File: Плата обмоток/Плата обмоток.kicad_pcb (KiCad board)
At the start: 2 copper layers, 58 x 58 mm, 20 parts, among them J1 4900, J10 4900, J11 4900, J12 4900, J13 4900, J14 A1, J15 A2, J16 B1, J17 B2, J18 C1, J19 C2, J2 4900, J3 4900, J4 Conn_01x02, J5 Conn_02x02_Odd_Even, J6 Conn_01x02, J7 Conn_01x02, J8 4900, J9 4900

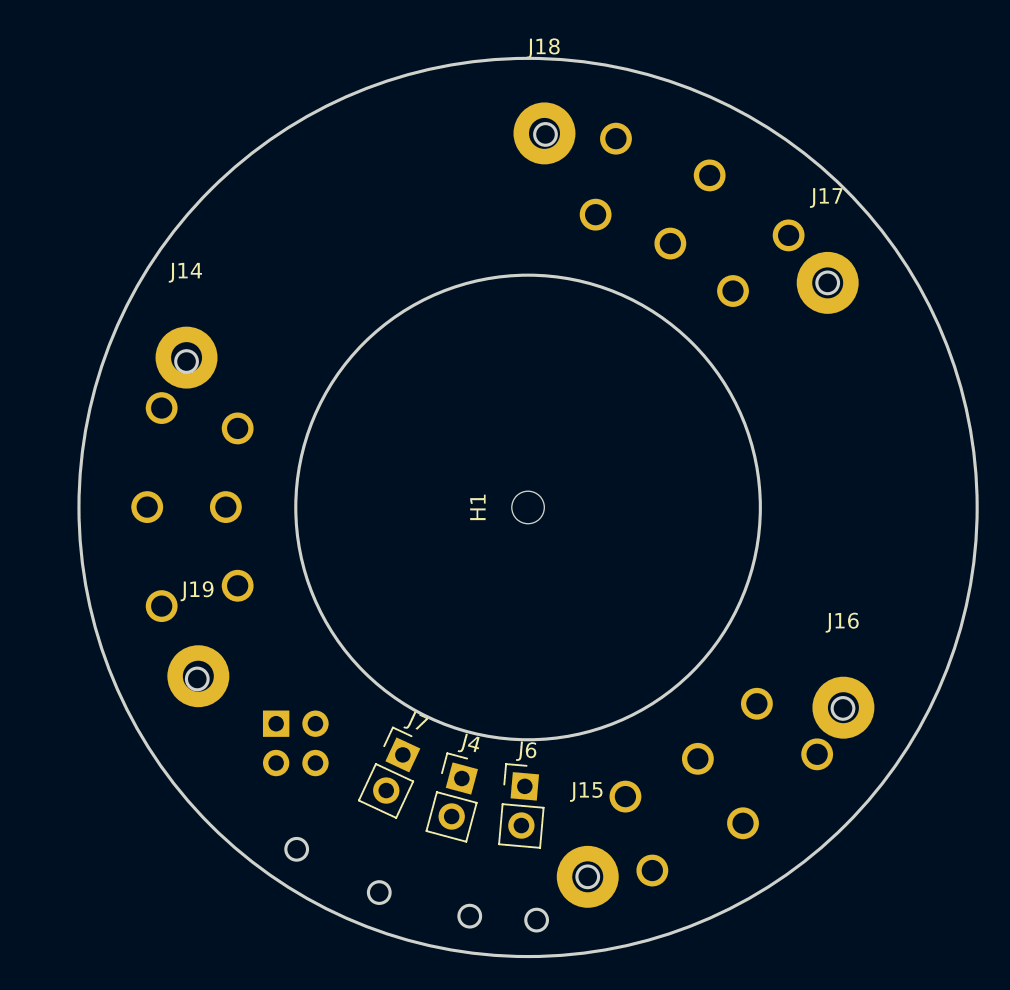
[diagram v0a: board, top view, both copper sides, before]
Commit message: Финальная доработка
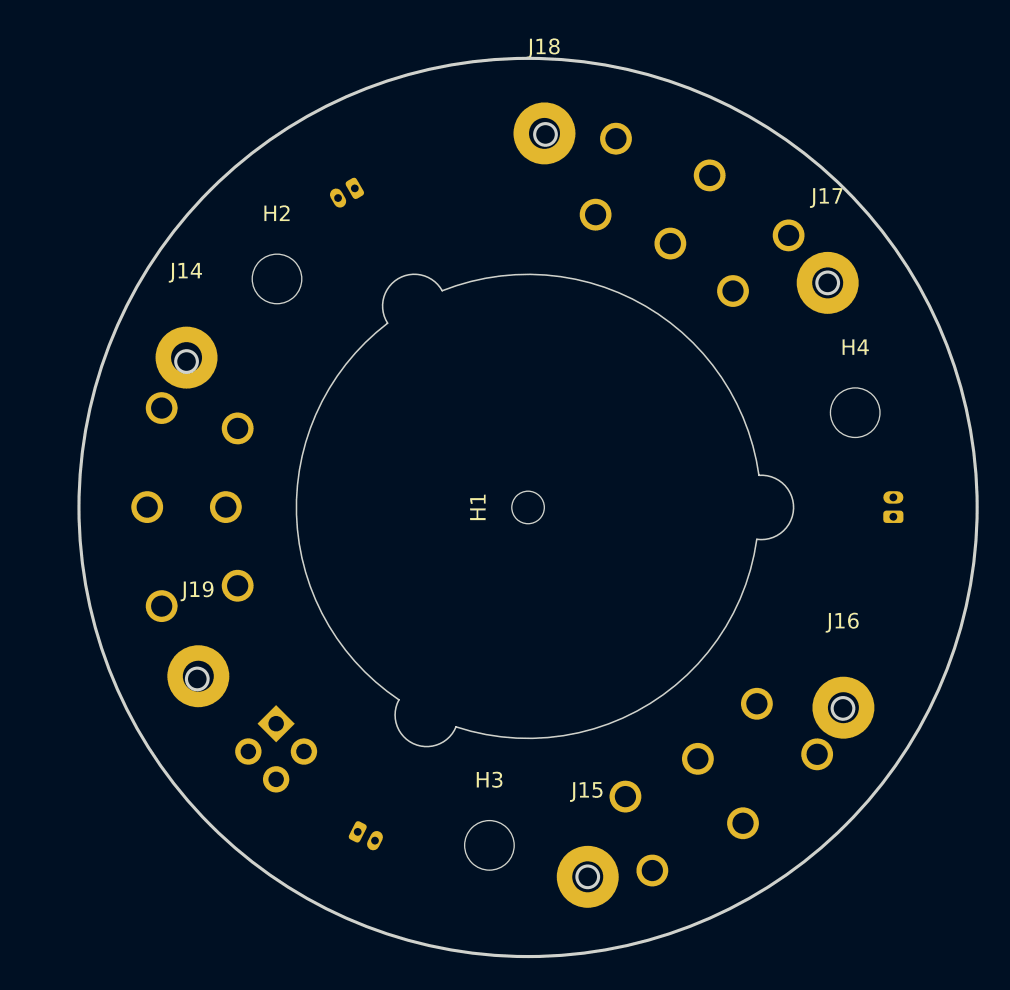
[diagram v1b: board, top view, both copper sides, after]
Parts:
- added H2: MountingHole, MountingHole:MountingHole_3.2mm_M3, F.Cu at (67.1, 81.3)
- added H3: MountingHole, MountingHole:MountingHole_3.2mm_M3, F.Cu at (80.8, 117.9)
- added H4: MountingHole, MountingHole:MountingHole_3.2mm_M3, F.Cu at (104.4, 89.9)
- J4, J6, J7: footprint Connector_PinHeader_2.54mm:PinHeader_1x02_P2.54mm_Vertical -> Connector_Molex:Molex_PicoBlade_53048-0210_1x02_P1.25mm_Horizontal; moved to B.Cu
- moved J6 40.1 mm to (72.1, 75.4), turned to -150 degrees
- moved J4 32.6 mm to (106.9, 96.6), turned to 90 degrees
- moved J7 5.76 mm to (72.3, 117.0), turned to -27 degrees
- turned J5 to 135 degrees
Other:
- outline, holes or cut-outs redrawn

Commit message: Ещё доработать
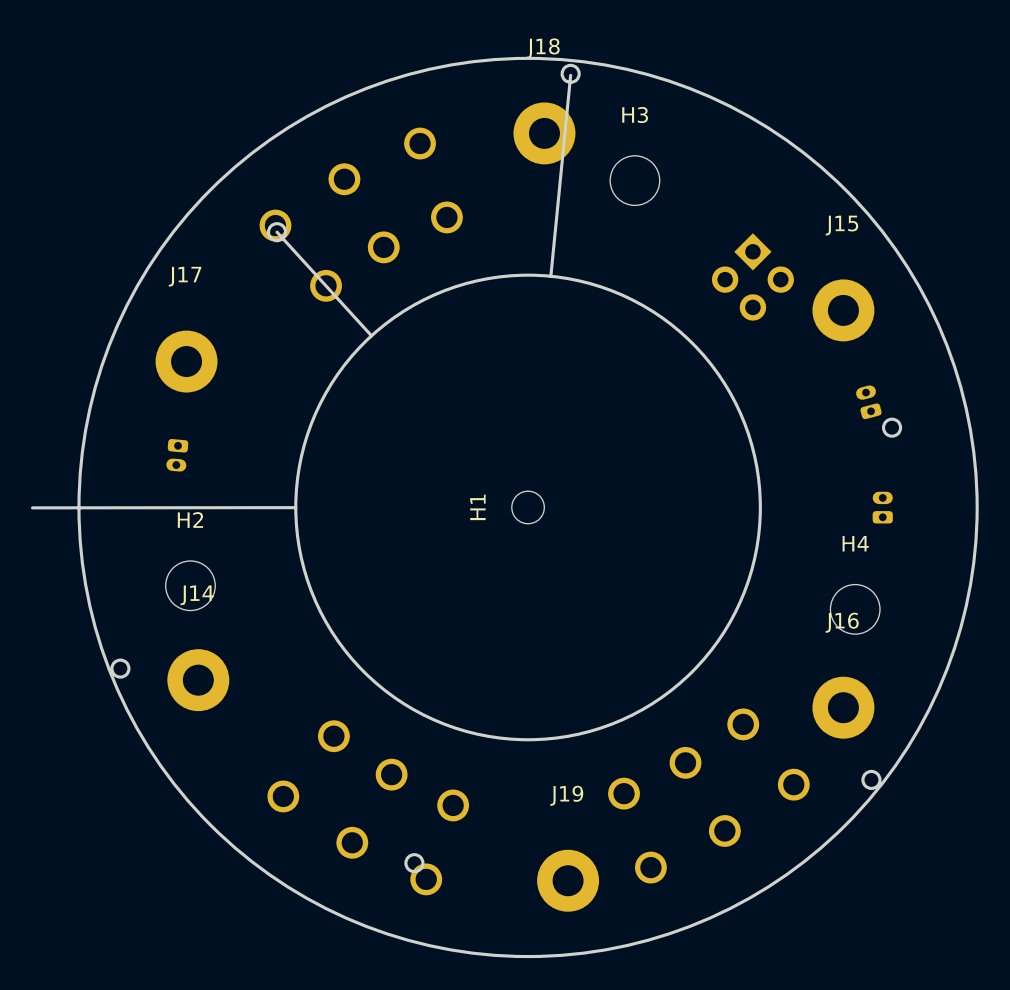
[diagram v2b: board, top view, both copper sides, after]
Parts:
- moved H3 43.9 mm to (90.2, 74.9)
- moved J9 43.8 mm to (71.9, 117.7)
- moved J5 43.3 mm to (97.8, 79.5)
- moved J8 42.8 mm to (76.7, 120.1), turned to 70 degrees
- moved J10 42.6 mm to (67.5, 114.7), turned to 50 degrees
- moved J17 41.7 mm to (61.2, 86.6)
- moved J15 40.1 mm to (103.6, 83.3)
- moved J6 36.3 mm to (105.4, 89.8), turned to 105 degrees
- moved J7 27.5 mm to (60.7, 92.1), turned to -95 degrees
- moved J19 27.3 mm to (85.9, 120.1)
- moved J11 25.6 mm to (67.0, 77.8), turned to -50 degrees
- moved J12 24.7 mm to (71.4, 74.8), turned to -60 degrees
- moved J13 23.9 mm to (76.3, 72.5), turned to -70 degrees
- moved J14 20.8 mm to (62.0, 107.2)
- moved H2 20.6 mm to (61.5, 101.1)
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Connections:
- J10 pad 1: B_OUT -> C_OUT
- J10 pad 2: B_OUT -> C_OUT
- J11 pad 1: C_OUT -> B_OUT
- J11 pad 2: C_OUT -> B_OUT
- J12 pad 1: C_OUT -> B_OUT
- J12 pad 2: C_OUT -> B_OUT
- J13 pad 1: C_OUT -> B_OUT
- J13 pad 2: C_OUT -> B_OUT
- J8 pad 1: B_OUT -> C_OUT
- J8 pad 2: B_OUT -> C_OUT
- J9 pad 1: B_OUT -> C_OUT
- J9 pad 2: B_OUT -> C_OUT
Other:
- board size 58 x 58 mm -> 61 x 58 mm

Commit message: Собираю документацию
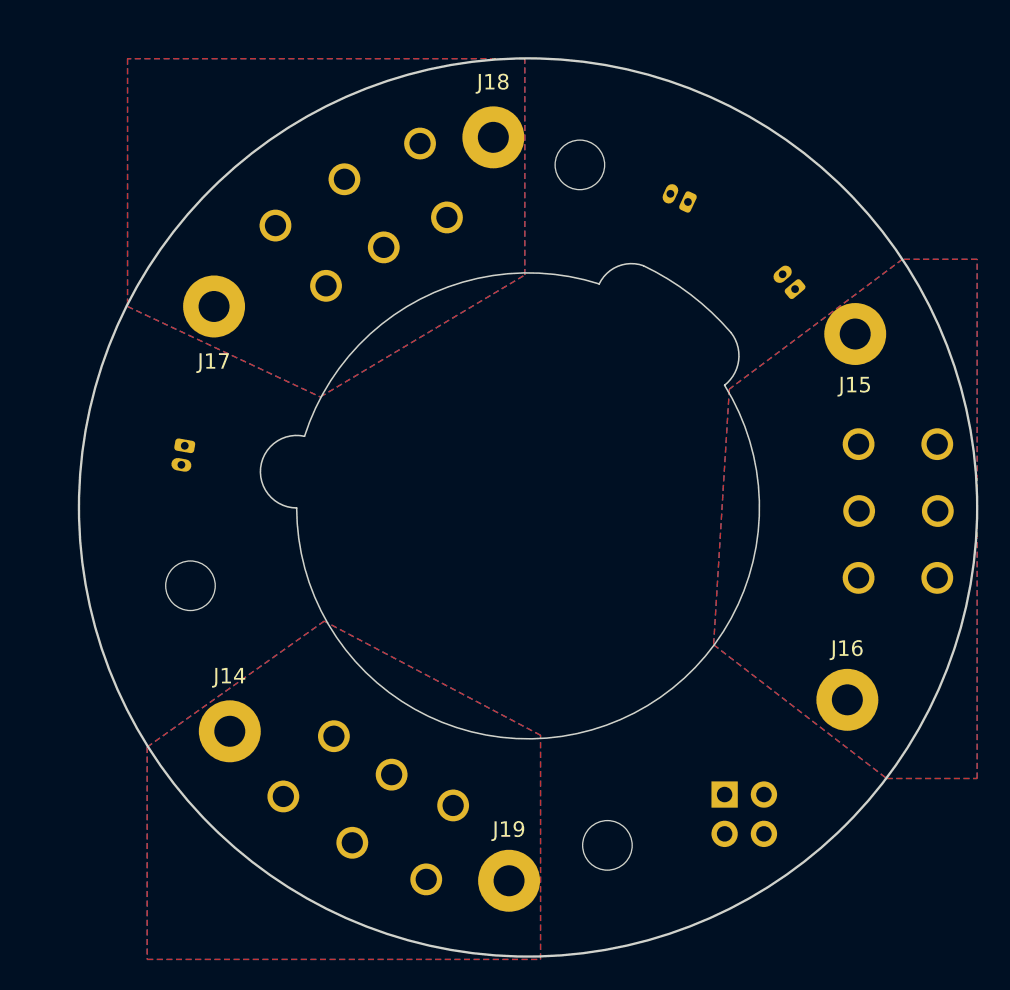
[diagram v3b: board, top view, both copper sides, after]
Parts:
- removed H1: MountingHole, MountingHole:MountingHole_2.1mm
- moved J5 35.1 mm to (96.0, 114.6), turned to 180 degrees
- moved J1 26.3 mm to (109.7, 100.6), turned to 180 degrees
- moved J4 23.9 mm to (93.6, 76.3), turned to 155 degrees
- moved J3 23.9 mm to (109.7, 91.9), turned to 180 degrees
- moved J2 22.4 mm to (104.6, 96.3), turned to 0 degrees
- moved H4 22.1 mm to (88.4, 117.9)
- moved J6 9.29 mm to (100.5, 81.9), turned to 130 degrees
- moved J17 3.98 mm to (63.0, 83.1)
- moved J14 3.88 mm to (64.0, 110.5)
- moved J19 3.81 mm to (82.0, 120.1)
- moved H3 3.70 mm to (86.6, 73.9)
- moved J18 3.31 mm to (81.0, 72.1)
- moved J15 1.70 mm to (104.4, 84.8)
- moved J16 0.57 mm to (103.9, 108.5)
- moved J7 0.43 mm to (61.1, 92.1), turned to -100 degrees
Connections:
- J5 pad 2: PTC_Coil_C -> GNDA
- J5 pad 3: PTC_Coil_B -> PTC_Coil_C
- J5 pad 4: GNDA -> PTC_Coil_B
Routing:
- net PTC_Coil_C: track 0.00 -> 48.2 mm
- net PTC_Coil_A: track 0.00 -> 42.4 mm
- net PTC_Coil_B: track 0.00 -> 36.3 mm
- added copper zone on B.Cu, net A_OUT
- added copper zone on F.Cu, net A_OUT
- added copper zone on B.Cu, net B_OUT
- added copper zone on F.Cu, net B_OUT
- added copper zone on B.Cu, net C_OUT
- added copper zone on F.Cu, net C_OUT
- added copper zone on In2.Cu, net GNDA
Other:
- board size 61 x 58 mm -> 58 x 58 mm
- copper layers 2 -> 4
- board text removed: "1"
- board text removed: "3"
